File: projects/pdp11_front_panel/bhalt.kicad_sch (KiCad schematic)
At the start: 6 parts

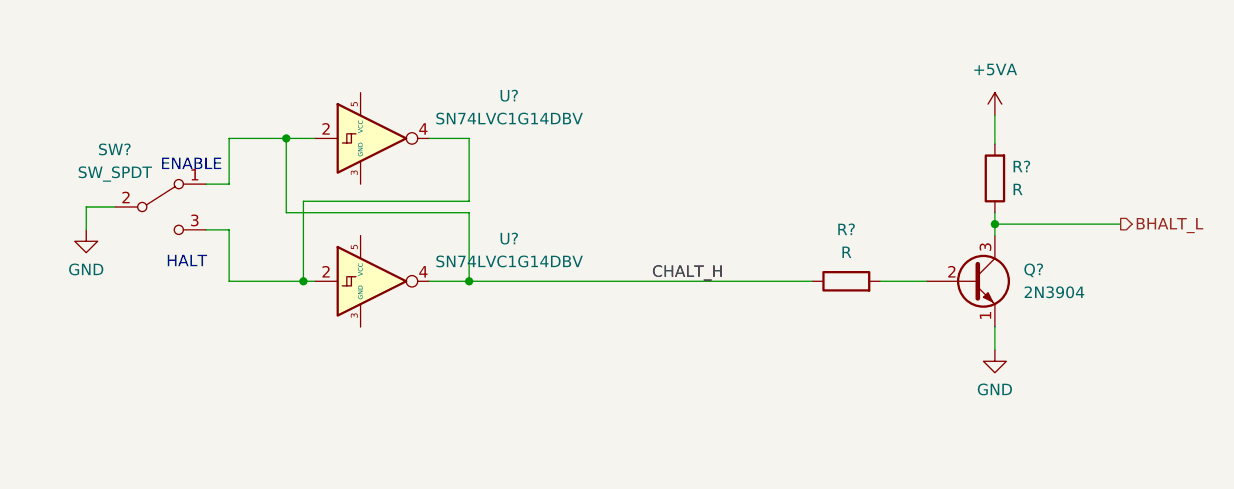
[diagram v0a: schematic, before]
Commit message: .
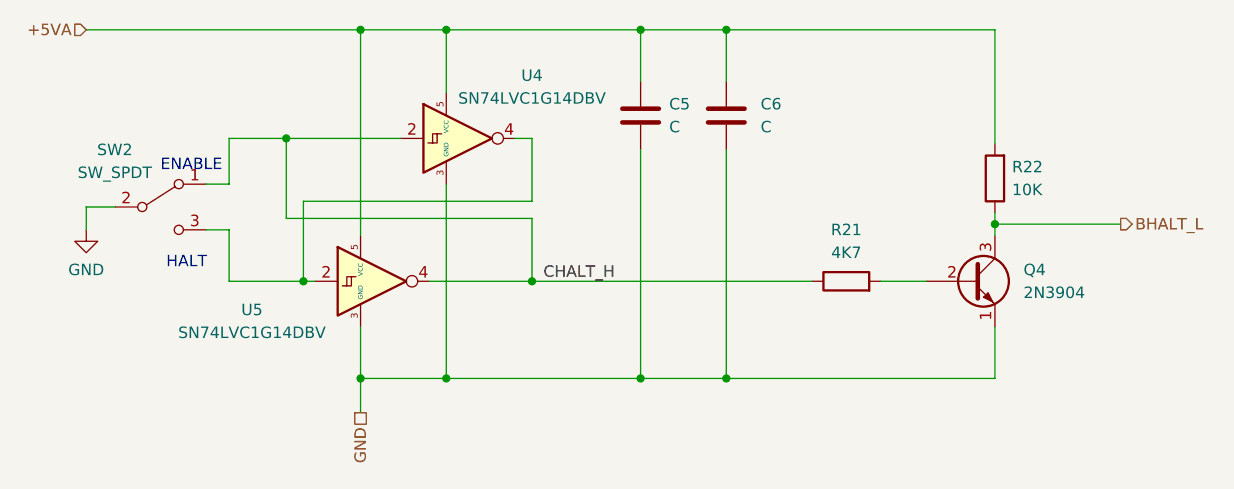
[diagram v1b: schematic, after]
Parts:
- added C5, C6: C, symbol Device:C
- R21: renamed from R?; value R -> 4K7
- R22: renamed from R?; value R -> 10K
- gave numbers to parts that had none: 4
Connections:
- net +5VA: now also U4.5 (VCC), U5.5 (VCC), C5.1, C6.1
- net GND: now also U4.3 (GND), U5.3 (GND), C5.2, C6.2
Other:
- moved on the sheet: U4
